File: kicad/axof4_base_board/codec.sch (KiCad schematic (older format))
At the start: 46 parts, among them J1 CLK_OUT, U1 CODECODER-WM8731SEDS_V(SSOP28), Y1 12.288MHz

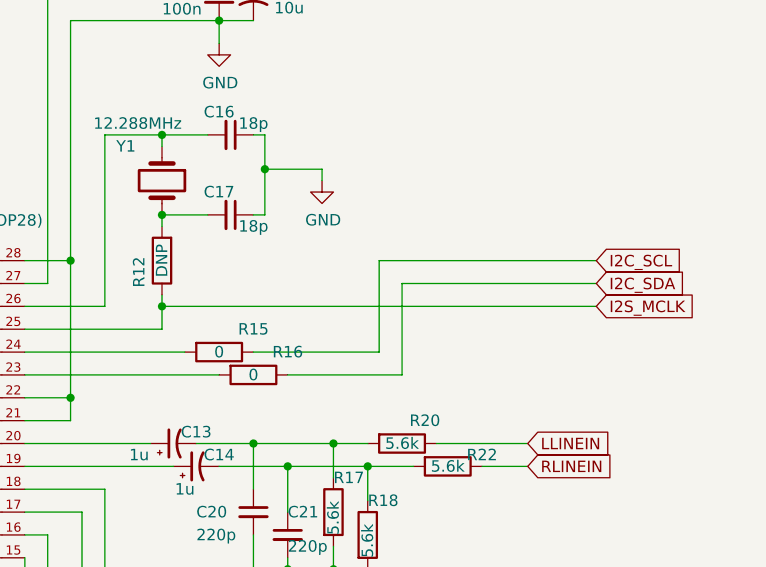
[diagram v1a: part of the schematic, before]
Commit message: kicad pcb backup, hohum axoctrl study
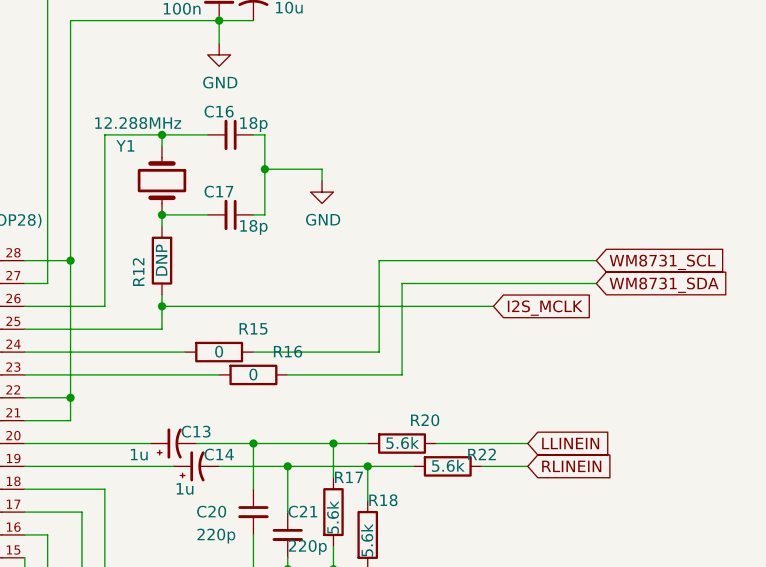
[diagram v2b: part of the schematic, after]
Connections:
- net I2C_SCL renamed WM8731_SCL
- net I2C_SDA renamed WM8731_SDA
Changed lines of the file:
@@
 RLINEIN
 Text GLabel 8900 2800 2    50   Input ~ 0
-I2C_SCL
+WM8731_SCL
 Text GLabel 8900 2900 2    50   Input ~ 0
-I2C_SDA
+WM8731_SDA
 $Comp
 L axof4_base_board-rescue:GNDA-power #PWR?
@@
 	-1   0    0    1
 $EndComp
-Text GLabel 8900 3000 2    50   Input ~ 0
+Text GLabel 8450 3000 2    50   Input ~ 0
 I2S_MCLK
 Wire Wire Line
-	7000 3000 8900 3000
+	7000 3000 8450 3000
 Wire Wire Line
 	4300 2550 4500 2550

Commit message: rollback kicad project to use STM32F4DISCOVERY
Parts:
- C1, C12, C19, C3, C5, C7, C9: footprint Capacitor_SMD:CP_Elec_4x5.4 -> Capacitor_SMD:CP_Elec_6.3x5.3
- C10, C11, C15, C16, C17, C2, C20, C21, C22, C8: footprint Capacitor_SMD:C_1206_3216Metric_Pad1.42x1.75mm_HandSolder -> Capacitor_SMD:C_0603_1608Metric
- R1, R10, R11, R12, R13, R14, R15, R16, R17, R18, R19, R2, R20, R22, R3, R4, R5, R6, R7, R8, R9: footprint Resistor_SMD:R_1206_3216Metric_Pad1.42x1.75mm_HandSolder -> Resistor_SMD:R_0603_1608Metric
- Y1: footprint Crystal:Crystal_HC49-U_Vertical -> Crystal:Crystal_SMD_HC49-SD

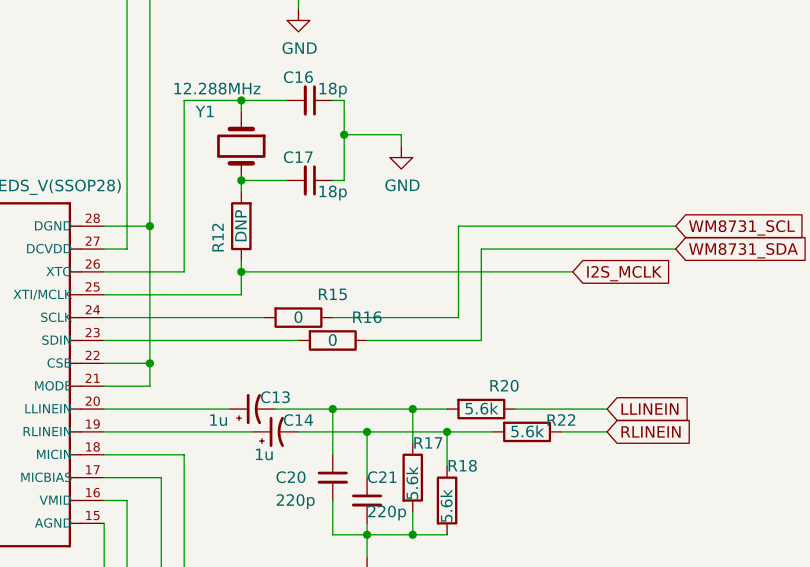
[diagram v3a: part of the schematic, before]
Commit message: blender edits
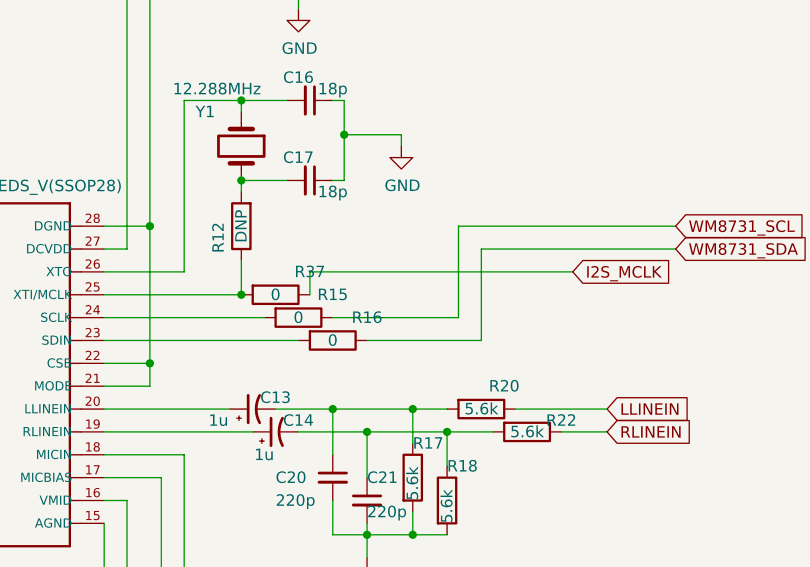
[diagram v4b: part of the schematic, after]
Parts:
- added R37: 0, Resistor_SMD:R_0603_1608Metric, symbol axof4_base_board-rescue:R-Device
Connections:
- net I2S_MCLK: now also R37.1; no longer R12.1, U1.25 (XTI/MCLK)
- new net: R12.1, R37.2, U1.25 (XTI/MCLK)
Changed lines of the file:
@@
 	7000 2650 7000 2600
 Connection ~ 7000 2600
-Wire Wire Line
-	7000 3100 7000 3000
-Connection ~ 7000 3000
-Wire Wire Line
-	7000 3000 7000 2950
 Text GLabel 4150 3000 0    50   Input ~ 0
 I2S_BCLK
@@
 I2S_MCLK
 Wire Wire Line
-	7000 3000 8450 3000
-Wire Wire Line
 	4300 2550 4500 2550
 Wire Wire Line
@@
 Text Notes 1100 1600 0    50   ~ 0
 Analog and digital GND are the same, \njust keeping different symbols for future upgrades
+Wire Wire Line
+	7000 2950 7000 3100
+$Comp
+L axof4_base_board-rescue:R-Device R?
+U 1 1 61619D0F
+P 7150 3100
+AR Path="/61619D0F" Ref="R?"  Part="1"
+AR Path="/5EFC127A/61619D0F" Ref="R37"  Part="1"
+F 0 "R37" V 7050 3250 50  0000 C CNN
+F 1 "0" V 7150 3100 50  0000 C CNN
+F 2 "Resistor_SMD:R_0603_1608Metric" V 7080 3100 50  0001 C CNN
+F 3 "~" H 7150 3100 50  0001 C CNN
+	1    7150 3100
+	0    1    1    0
+$EndComp
+Connection ~ 7000 3100
+Wire Wire Line
+	7300 3100 7300 3000
+Wire Wire Line
+	7300 3000 8450 3000
 $EndSCHEMATC
